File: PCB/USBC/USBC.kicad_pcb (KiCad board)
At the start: 2 copper layers, 70 x 70 mm, 29 parts, among them J1 USB-C-Plug-V, J2 Shelly, J3 USB-PROG, J4 Conn_01x03_Socket, U1 VEML6040, U2 ESP32-S3-MINI-1, U5 MD8942

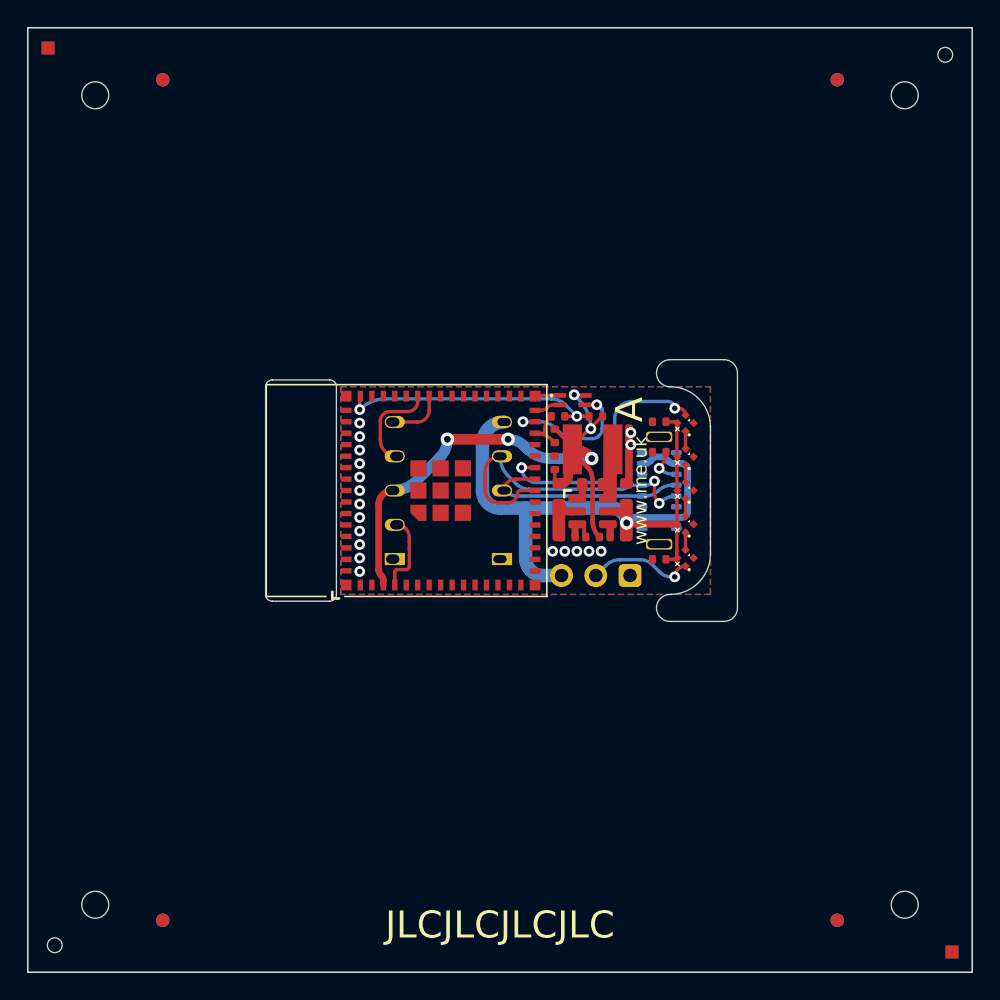
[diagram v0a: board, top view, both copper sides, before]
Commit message: New
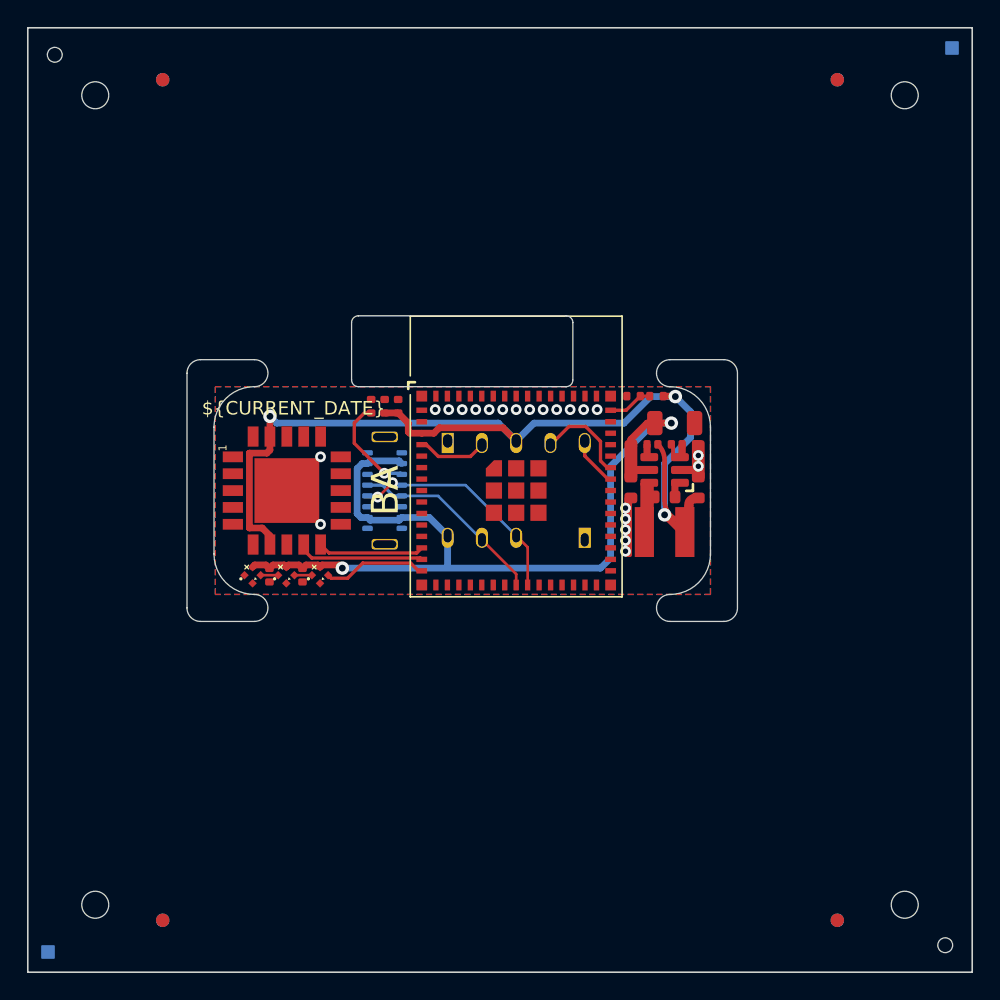
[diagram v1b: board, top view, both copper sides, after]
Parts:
- removed D4, D5: XL-1010RGBC-WS2812B, RevK:SMD1010
- removed J4: Conn_01x03_Socket, RevK:PinHeader_1x03_P2.54mm
- removed U1: VEML6040, RevK:VEML6040
- added C10: 100uF 6.3V, RevK:C_1206, F.Cu at (113.0, 94.3)
- added U3: SCD41, RevK:SCD41, F.Cu at (84.2, 99.3)
- PCB1: moved to B.Cu
- V1, V2: moved to F.Cu
- moved D3 32.7 mm to (81.7, 105.6), turned to 45 degrees
- moved D2 30.9 mm to (84.2, 105.6), turned to 45 degrees
- moved D1 29.3 mm to (86.7, 105.6), turned to 45 degrees
- moved C5 28.9 mm to (82.9, 105.6), turned to -90 degrees
- moved C4 28.8 mm to (85.4, 105.6), turned to -90 degrees
- moved R2 21.6 mm to (90.5, 93.0), turned to 90 degrees
- moved J1 20.3 mm to (91.5, 99.3)
- moved C2 12.8 mm to (91.5, 93.0), turned to 90 degrees
- moved C1 12.3 mm to (92.5, 93.0)
- moved R10 11.1 mm to (113.8, 95.9), turned to 0 degrees
- moved C7 10.2 mm to (114.5, 99.1), turned to -90 degrees
- moved J2 9.67 mm to (101.2, 95.8), turned to 180 degrees
- moved R9 8.57 mm to (112.0, 95.9), turned to 0 degrees
- moved L2 8.03 mm to (112.0, 102.4), turned to 0 degrees
- moved R11 7.02 mm to (110.2, 95.9), turned to 0 degrees
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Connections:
- D3 pad 1: Net-(D3-O) -> unconnected-(D3-O-Pad1)
- U2 pad 13: unconnected-(U2-GPIO9-Pad13) -> SDA
- U2 pad 14: unconnected-(U2-GPIO10-Pad14) -> SCL
- U2 pad 15: unconnected-(U2-GPIO11-Pad15) -> LED
- U2 pad 25: LED -> unconnected-(U2-GPIO21-Pad25)
- U2 pad 29: SCL -> unconnected-(U2-GPIO34-Pad29)
- U2 pad 30: SDA -> unconnected-(U2-GPIO48-Pad30)
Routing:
- net +3.3V: track 35.9 -> 68.5 mm, vias 5 -> 3
- net Net-(U2-EN): track 20.4 -> 3.33 mm, vias 2 -> 0
- net LED: track 19.5 -> 7.74 mm, vias 2 -> 0
- net VBUS: track 52.2 -> 62.2 mm, vias 1 -> 2
- net D-: track 23.9 -> 15.0 mm, vias 2 -> 0
- net Net-(D5-O): track 7.90 -> 0.00 mm, vias 1 -> 0
- net SDA: track 1.95 -> 7.91 mm
- net GND: track 5.56 -> 0.00 mm, vias 19 -> 22
- net Net-(J1-CC): track 2.71 -> 7.53 mm
- net Net-(D3-O): track 1.40 -> 0.00 mm
- net D+: track 15.8 -> 17.1 mm, vias 0 -> 2
- net Net-(D4-O): track 1.30 -> 0.00 mm
- net SCL: track 10.4 -> 9.44 mm, vias 2 -> 0
- net Net-(J2-0): track 5.85 -> 5.17 mm
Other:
- board text added: "AB"
- board text added: "BA"
- board text added: "CO₂"
- board text added: "SDA:9 SCL:10 RGB:11"
- board text removed: "5060634238137"
- board text removed: "A"
- board text removed: "B"
- board text removed: "RGB:21"
- board text removed: "SCL:34 SDA:48"
- board text removed: "USB-C"
- board text removed: "usbc.revk.uk"
- board text removed: "www.me.uk"
- board text removed: "⏚"
